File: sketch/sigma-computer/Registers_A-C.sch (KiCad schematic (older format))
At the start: 12 parts

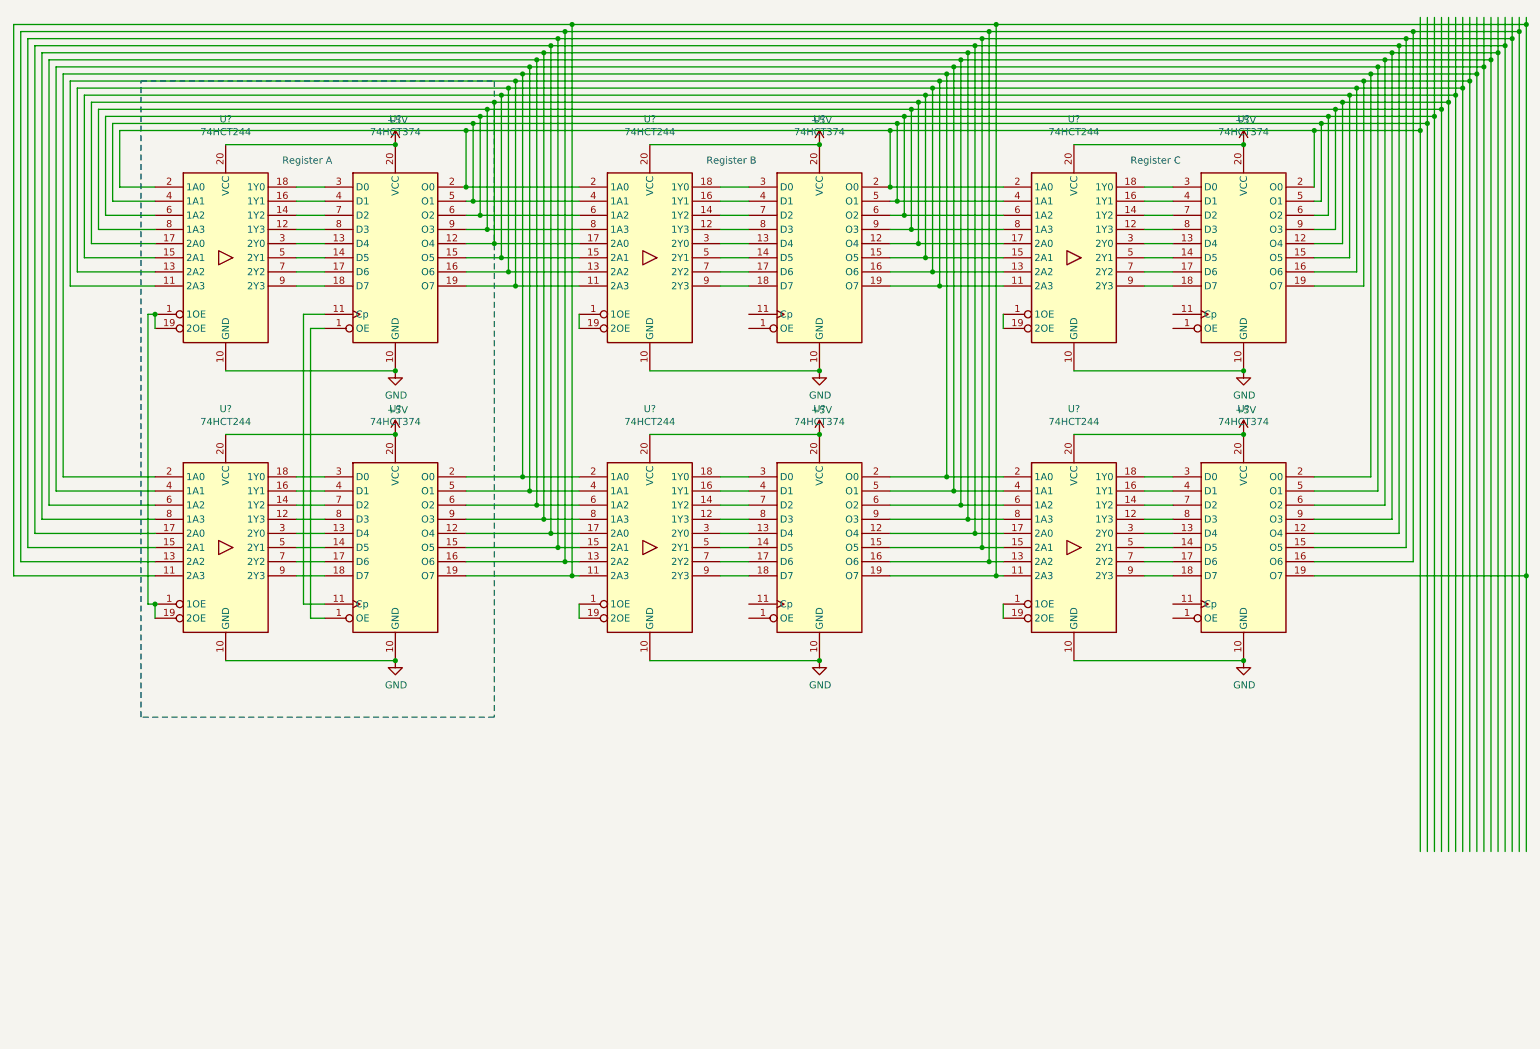
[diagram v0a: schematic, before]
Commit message: Changes in the schematic
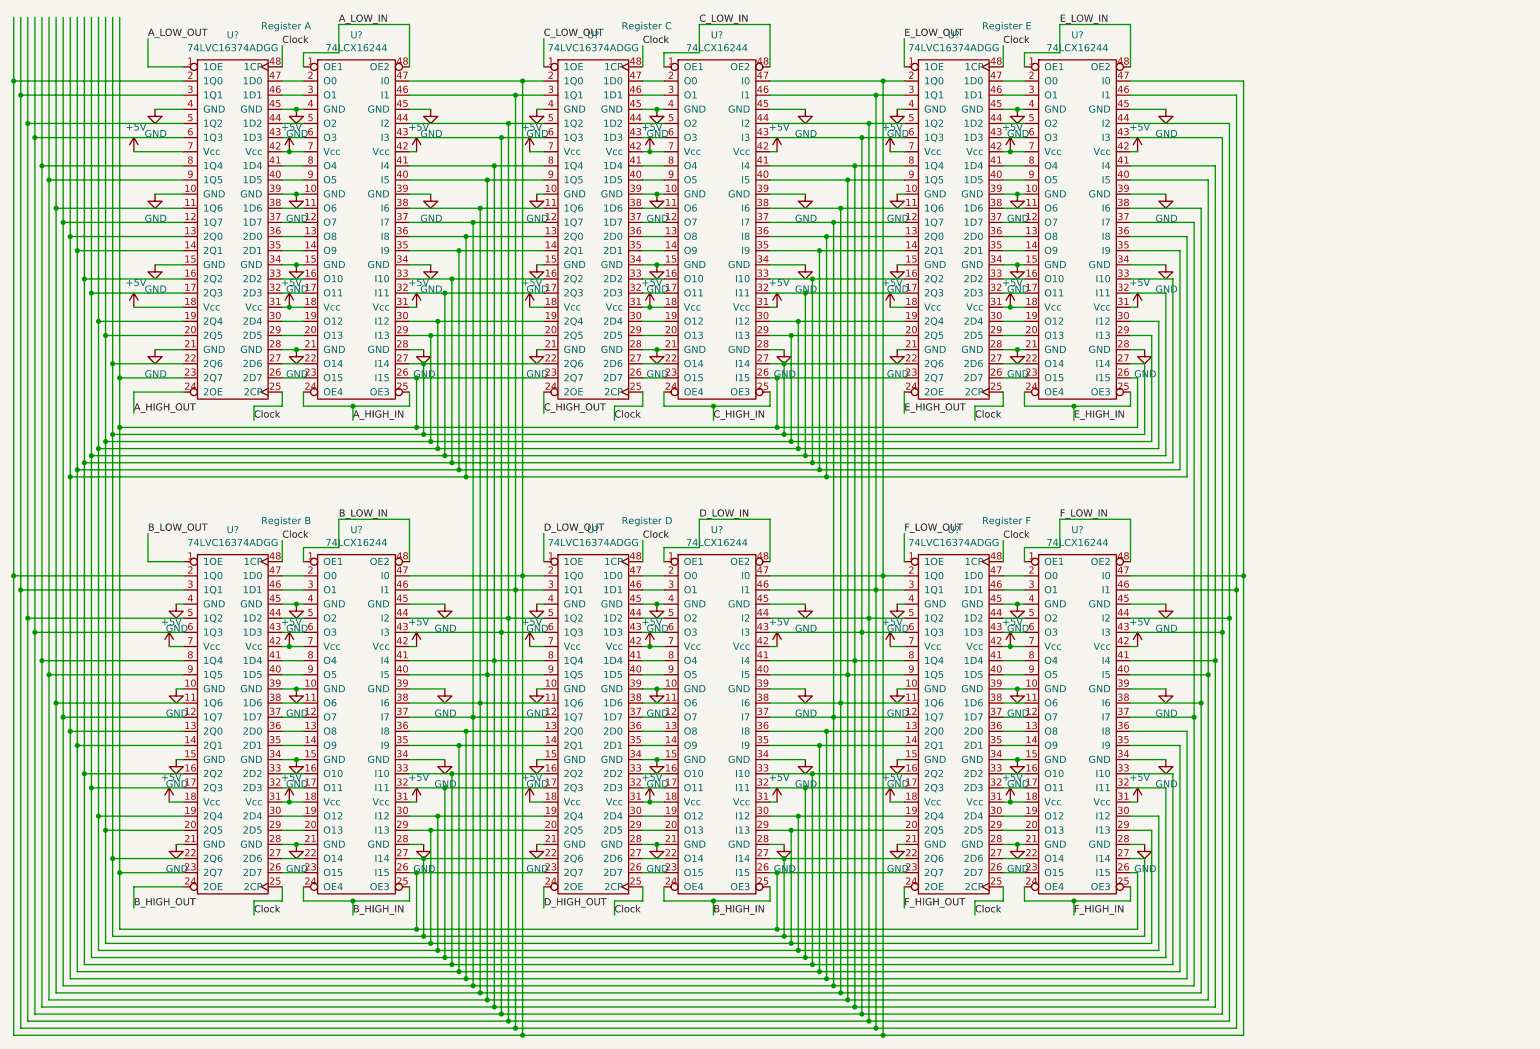
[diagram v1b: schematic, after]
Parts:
- removed U? (x6): 74HCT374, symbol 74xx:74HCT374
- removed U? (x6): 74HCT244, symbol 74xx:74HCT244
- added U? (x6): 74LVC16374ADGG, symbol Additional74:74LVC16374ADGG
- added U? (x6): 74LCX16244, symbol Additional74:74LCX16244
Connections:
- net labels added: A_HIGH_IN, A_HIGH_OUT, A_LOW_IN, A_LOW_OUT, B_HIGH_IN, B_HIGH_OUT, B_LOW_IN, B_LOW_OUT, C_HIGH_IN, C_HIGH_OUT, C_LOW_IN, C_LOW_OUT, Clock, D_HIGH_OUT, D_LOW_IN, D_LOW_OUT, E_HIGH_IN, E_HIGH_OUT, E_LOW_IN, E_LOW_OUT, F_HIGH_IN, F_HIGH_OUT, F_LOW_IN, F_LOW_OUT
- wire segments 327 -> 760
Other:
- note added: "Register A\n"
- note added: "Register B\n"
- note added: "Register C\n"
- note added: "Register D\n"
- note added: "Register E"
- note added: "Register F\n"
- note removed: "Register A"
- note removed: "Register B"
- note removed: "Register C"
